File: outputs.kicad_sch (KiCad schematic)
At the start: 13 parts, among them Q1 CSD17575Q3T, U2 MAX14922ATE+

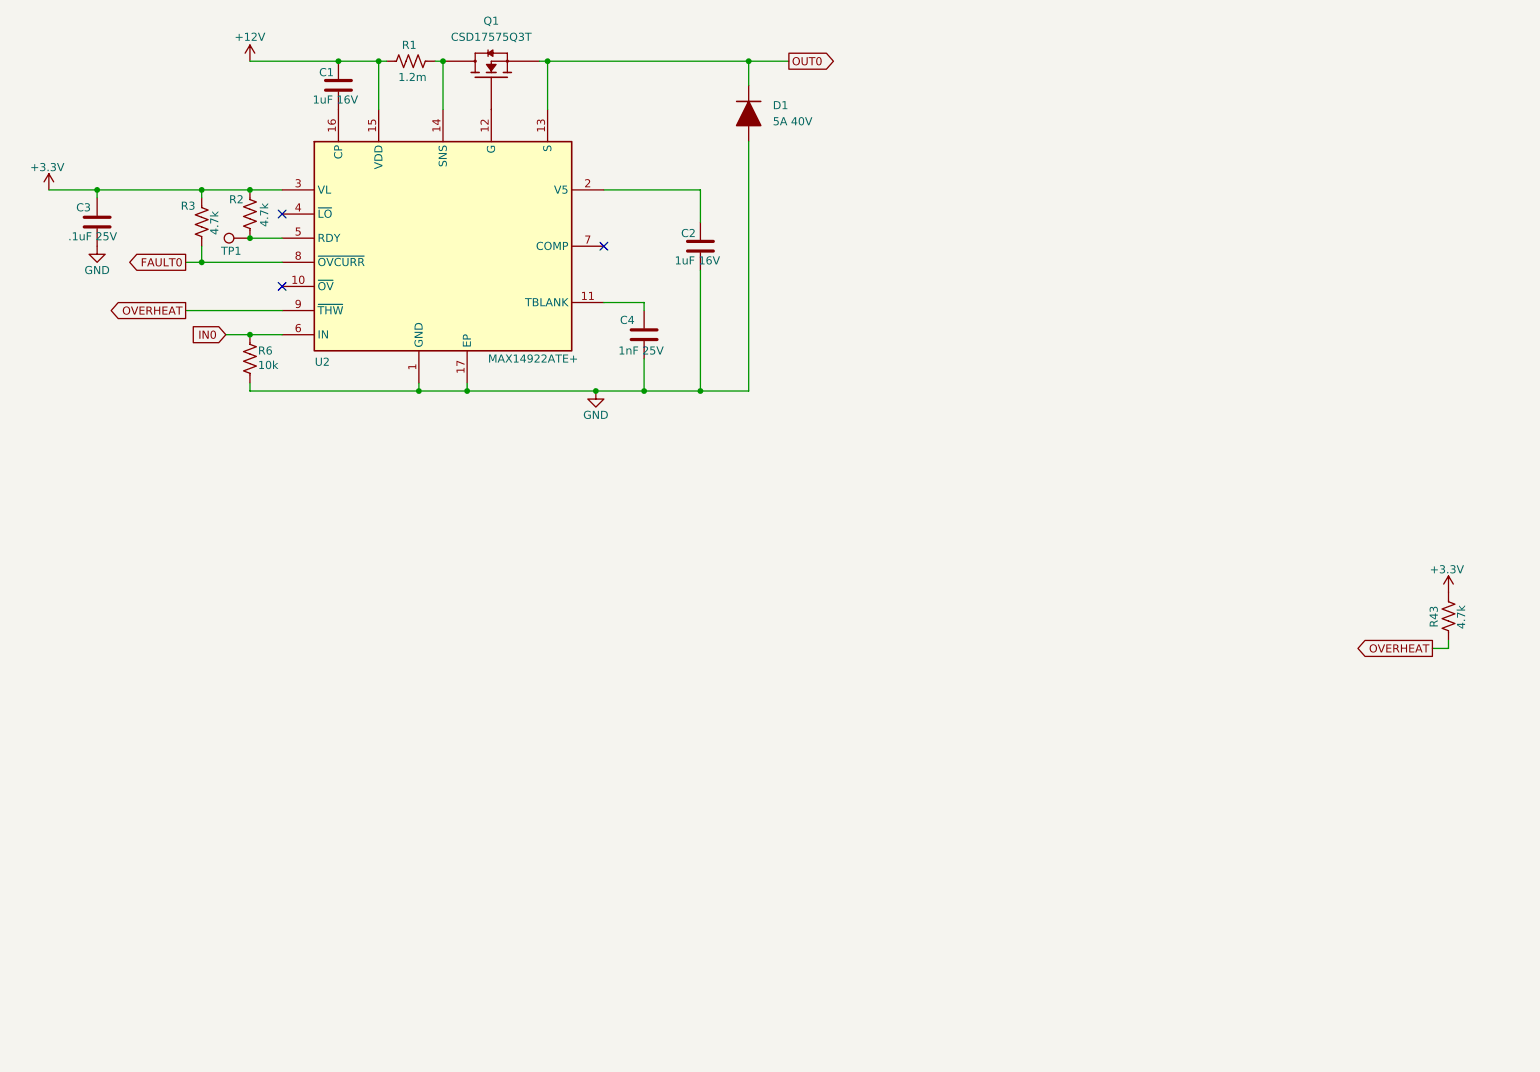
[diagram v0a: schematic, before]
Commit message: Initial schematic is done
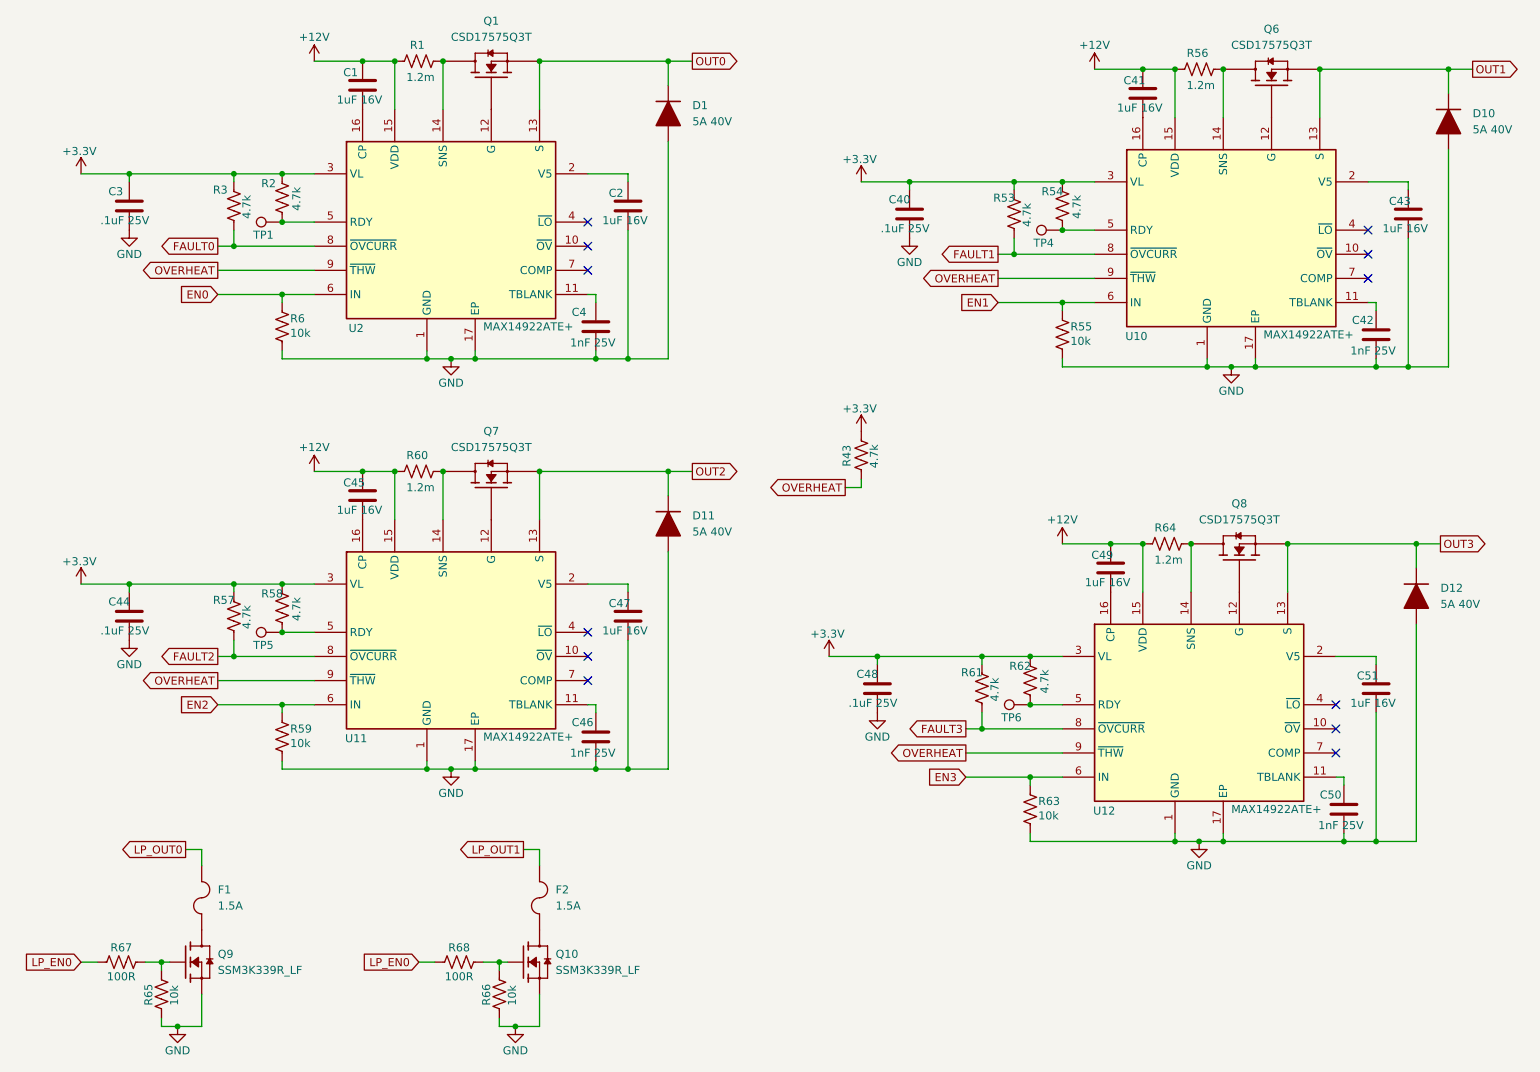
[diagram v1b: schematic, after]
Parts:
- added C40, C44, C48: .1uF 25V, Sullivan-Labs:C_0402_1005Metric, symbol Sullivan-Labs:CAP_.1uF_25V_0402
- added C41, C43, C45, C47, C49, C51: 1uF 16V, Sullivan-Labs:C_0402_1005Metric, symbol Sullivan-Labs:CAP_1uF_16V_0402
- added C42, C46, C50: 1nF 25V, Sullivan-Labs:C_0402_1005Metric, symbol Sullivan-Labs:CAP_1nF_25V_0402
- added D10, D11, D12: 5A 40V, Sullivan-Labs:DO-214AC, symbol Sullivan-Labs:DIODE 5A 40V Schottkey
- added F1, F2: 1.5A, Sullivan-Labs:FUSC1608X56N, symbol Sullivan-Labs:FUSE 1.5A Fast Blow
- added Q10, Q9: SSM3K339R_LF, Sullivan-Labs:SOT-23F_TOS, symbol Sullivan-Labs:NMOS 40V 2A
- added Q6, Q7, Q8: CSD17575Q3T, Sullivan-Labs:TRANS_CSD17308Q3, symbol Sullivan-Labs:NMOS 60A 30V
- added R53, R54, R57, R58, R61, R62: 4.7k, Sullivan-Labs:R_0402_1005Metric, symbol Sullivan-Labs:RES_4.7k_0402
- added R55, R59, R63, R65, R66: 10k, Sullivan-Labs:R_0402_1005Metric, symbol Sullivan-Labs:RES_10k_0402
- added R56, R60, R64: 1.2m, Sullivan-Labs:R_2512_6332Metric_Pad1.40x3.35mm_HandSolder, symbol Sullivan-Labs:RES_1.2m_2512
- added R67, R68: 100R, Sullivan-Labs:R_0402_1005Metric, symbol Sullivan-Labs:RES_100R_0402
- added TP4, TP5, TP6: TestPoint, Sullivan-Labs:TestPoint_Pad_D1.0mm, symbol Sullivan-Labs:TP 1mm Circle
- added U10, U11, U12: MAX14922ATE+, Sullivan-Labs:QFN50P300X300X80-17N, symbol Sullivan-Labs:IC High Side Switch Ex FET
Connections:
- net +12V: now also C41.1, C45.1, C49.1, R56.1, R60.1, R64.1, U10.15 (VDD), U11.15 (VDD), U12.15 (VDD)
- net +3.3V: now also C40.1, C44.1, C48.1, R53.1, R54.1, R57.1, R58.1, R61.1, R62.1, U10.3 (VL), U11.3 (VL), U12.3 (VL)
- net GND: now also C40.2, C42.2, C43.2, C44.2, C46.2, C47.2, C48.2, C50.2, C51.2, D10.2 (A), D11.2 (A), D12.2 (A), Q10.2, Q9.2, R55.2, R59.2, R63.2, R65.2, R66.2, U10.1 (GND), U10.17 (EP), U11.1 (GND), U11.17 (EP), U12.1 (GND), U12.17 (EP)
- net OVERHEAT: now also U10.9 (~{THW}), U11.9 (~{THW}), U12.9 (~{THW})
- net IN0 renamed EN0
- new net: C51.1, U12.2 (V5)
- new net: C46.1, U11.11 (TBLANK)
- new net: Q8.4 (G), U12.12 (G)
- new net: Q8.5 (D), Q8.6 (D), Q8.7 (D), Q8.8 (D), Q8.9 (D), R64.2, U12.14 (SNS)
- new net: C50.1, U12.11 (TBLANK)
- new net: C49.2, U12.16 (CP)
- new net: R62.2, TP6.1, U12.5 (RDY)
- new net: F2.1, Q10.3
- new net: Q10.1, R66.1, R68.2
- new net: Q6.4 (G), U10.12 (G)
- new net: Q6.5 (D), Q6.6 (D), Q6.7 (D), Q6.8 (D), Q6.9 (D), R56.2, U10.14 (SNS)
- new net: R58.2, TP5.1, U11.5 (RDY)
- new net: R54.2, TP4.1, U10.5 (RDY)
- new net: C47.1, U11.2 (V5)
- new net: C43.1, U10.2 (V5)
- new net: C42.1, U10.11 (TBLANK)
- new net: Q7.4 (G), U11.12 (G)
- new net: Q7.5 (D), Q7.6 (D), Q7.7 (D), Q7.8 (D), Q7.9 (D), R60.2, U11.14 (SNS)
- new net: Q9.1, R65.1, R67.2
- new net: C41.2, U10.16 (CP)
- new net: C45.2, U11.16 (CP)
- new net: F1.1, Q9.3
- new net EN1: R55.1, U10.6 (IN)
- new net EN2: R59.1, U11.6 (IN)
- new net EN3: R63.1, U12.6 (IN)
- new net FAULT1: R53.2, U10.8 (~{OVCURR})
- new net FAULT2: R57.2, U11.8 (~{OVCURR})
- new net FAULT3: R61.2, U12.8 (~{OVCURR})
- new net LP_EN0: R67.1, R68.1
- new net LP_OUT0: F1.2
- new net LP_OUT1: F2.2
- new net OUT1: D10.1 (K), Q6.1 (S), Q6.2 (S), Q6.3 (S), U10.13 (S)
- new net OUT2: D11.1 (K), Q7.1 (S), Q7.2 (S), Q7.3 (S), U11.13 (S)
- new net OUT3: D12.1 (K), Q8.1 (S), Q8.2 (S), Q8.3 (S), U12.13 (S)
- no-connect marks 3 -> 12
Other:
- moved on the sheet: C1, C2, C3, C4, D1, R1, R2, R3, R43, R6, TP1, U2
